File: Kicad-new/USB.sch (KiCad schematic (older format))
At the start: 23 parts, among them J10 USB_C_Receptacle_USB2.0, J5 Relais, Q1 2N3904_SOT23, Q2 2N3904_SOT23, Q7 2N3904_SOT23, Q8 2N3904_SOT23, U4 CP2102N-A01-GQFN28

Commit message: new pcb
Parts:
- J10: symbol ESP32_TouchDown-rescue:USB_C_Receptacle_USB2.0-Connector -> ESP32Vfo:USB_C_Receptacle_USB2.0-Connector
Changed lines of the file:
@@
 $EndComp
 $Comp
-L ESP32_TouchDown-rescue:USB_C_Receptacle_USB2.0-Connector J?
+L ESP32Vfo:USB_C_Receptacle_USB2.0-Connector J?
 U 1 1 614D5451
 P 2550 1900

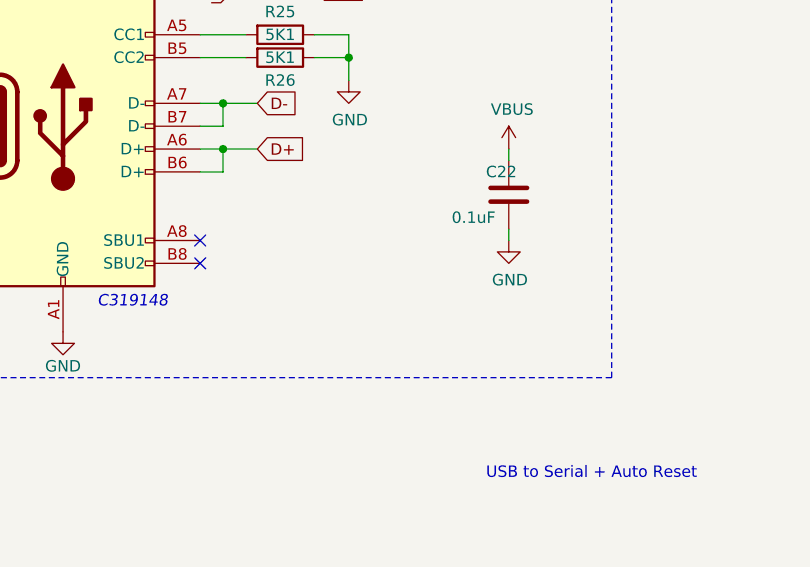
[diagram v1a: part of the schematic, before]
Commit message: update pcb
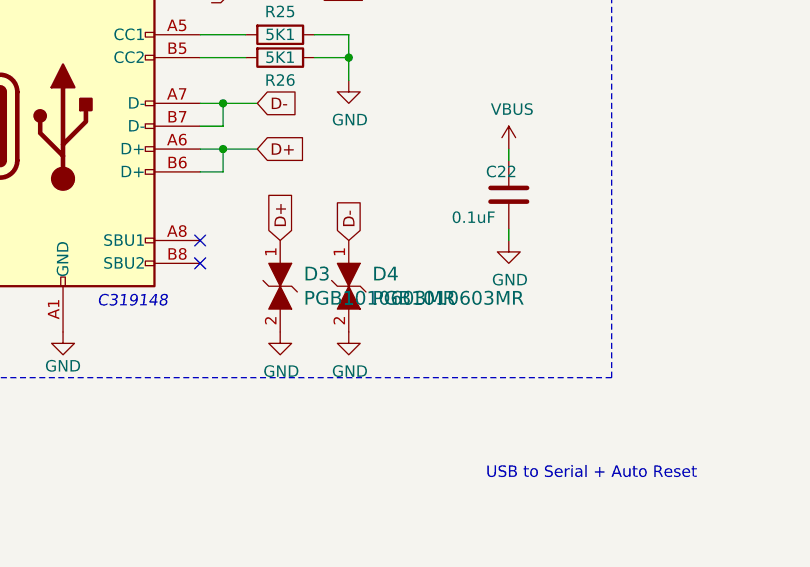
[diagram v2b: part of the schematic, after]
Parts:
- added D3, D4: PGB1010603MR, digikey-footprints:0603, symbol dk_TVS-Diodes:PGB1010603MR
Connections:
- net D+: now also D3.1
- net D-: now also D4.1
- net GND: now also D3.2, D4.2
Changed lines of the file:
@@
 Text GLabel 7750 4750 2    50   Input ~ 0
 IO0
+$Comp
+L power:GND #PWR?
+U 1 1 61918278
+P 3800 2800
+AR Path="/614AF034/61918278" Ref="#PWR?"  Part="1"
+AR Path="/614CC1BF/61918278" Ref="#PWR07"  Part="1"
+F 0 "#PWR07" H 3800 2550 50  0001 C CNN
+F 1 "GND" H 3805 2627 50  0000 C CNN
+F 2 "" H 3800 2800 50  0001 C CNN
+F 3 "" H 3800 2800 50  0001 C CNN
+	1    3800 2800
+	1    0    0    -1
+$EndComp
+$Comp
+L power:GND #PWR?
+U 1 1 6191868F
+P 3500 2800
+AR Path="/614AF034/6191868F" Ref="#PWR?"  Part="1"
+AR Path="/614CC1BF/6191868F" Ref="#PWR05"  Part="1"
+F 0 "#PWR05" H 3500 2550 50  0001 C CNN
+F 1 "GND" H 3505 2627 50  0000 C CNN
+F 2 "" H 3500 2800 50  0001 C CNN
+F 3 "" H 3500 2800 50  0001 C CNN
+	1    3500 2800
+	1    0    0    -1
+$EndComp
+Text GLabel 3800 2400 1    50   Input ~ 0
+D-
+Text GLabel 3500 2400 1    50   Input ~ 0
+D+
+$Comp
+L dk_TVS-Diodes:PGB1010603MR D3
+U 1 1 61994C49
+P 3500 2600
+F 0 "D3" V 3447 2703 60  0000 L CNN
+F 1 "PGB1010603MR" V 3553 2703 60  0000 L CNN
+F 2 "digikey-footprints:0603" H 3700 2800 60  0001 L CNN
+F 3 "https://www.littelfuse.com/data/en/data_sheets/littelfuse_pulseguard-esd_pgb1.pdf" H 3700 2900 60  0001 L CNN
+F 4 "F2594CT-ND" H 3700 3000 60  0001 L CNN "Digi-Key_PN"
+F 5 "PGB1010603MR" H 3700 3100 60  0001 L CNN "MPN"
+F 6 "Circuit Protection" H 3700 3200 60  0001 L CNN "Category"
+F 7 "TVS - Diodes" H 3700 3300 60  0001 L CNN "Family"
+F 8 "https://www.littelfuse.com/data/en/data_sheets/littelfuse_pulseguard-esd_pgb1.pdf" H 3700 3400 60  0001 L CNN "DK_Datasheet_Link"
+F 9 "/product-detail/en/littelfuse-inc/PGB1010603MR/F2594CT-ND/813072" H 3700 3500 60  0001 L CNN "DK_Detail_Page"
+F 10 "TVS DIODE 24V 150V 0603" H 3700 3600 60  0001 L CNN "Description"
+F 11 "Littelfuse Inc." H 3700 3700 60  0001 L CNN "Manufacturer"
+F 12 "Active" H 3700 3800 60  0001 L CNN "Status"
+	1    3500 2600
+	0    1    1    0
+$EndComp
+$Comp
+L dk_TVS-Diodes:PGB1010603MR D4
+U 1 1 6199685E
+P 3800 2600
+F 0 "D4" V 3747 2703 60  0000 L CNN
+F 1 "PGB1010603MR" V 3853 2703 60  0000 L CNN
+F 2 "digikey-footprints:0603" H 4000 2800 60  0001 L CNN
+F 3 "https://www.littelfuse.com/data/en/data_sheets/littelfuse_pulseguard-esd_pgb1.pdf" H 4000 2900 60  0001 L CNN
+F 4 "F2594CT-ND" H 4000 3000 60  0001 L CNN "Digi-Key_PN"
+F 5 "PGB1010603MR" H 4000 3100 60  0001 L CNN "MPN"
+F 6 "Circuit Protection" H 4000 3200 60  0001 L CNN "Category"
+F 7 "TVS - Diodes" H 4000 3300 60  0001 L CNN "Family"
+F 8 "https://www.littelfuse.com/data/en/data_sheets/littelfuse_pulseguard-esd_pgb1.pdf" H 4000 3400 60  0001 L CNN "DK_Datasheet_Link"
+F 9 "/product-detail/en/littelfuse-inc/PGB1010603MR/F2594CT-ND/813072" H 4000 3500 60  0001 L CNN "DK_Detail_Page"
+F 10 "TVS DIODE 24V 150V 0603" H 4000 3600 60  0001 L CNN "Description"
+F 11 "Littelfuse Inc." H 4000 3700 60  0001 L CNN "Manufacturer"
+F 12 "Active" H 4000 3800 60  0001 L CNN "Status"
+	1    3800 2600
+	0    1    1    0
+$EndComp
 $EndSCHEMATC
